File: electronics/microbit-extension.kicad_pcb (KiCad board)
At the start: 2 copper layers, 55.9 x 63.5 mm, 29 parts, among them J1 microbit_edge_connector, SW1 SW_DIP_x01, SW2 SW_DIP_x01, SW3 SW_DIP_x01, SW4 SW_DIP_x01, U1 LD1117S33CTR

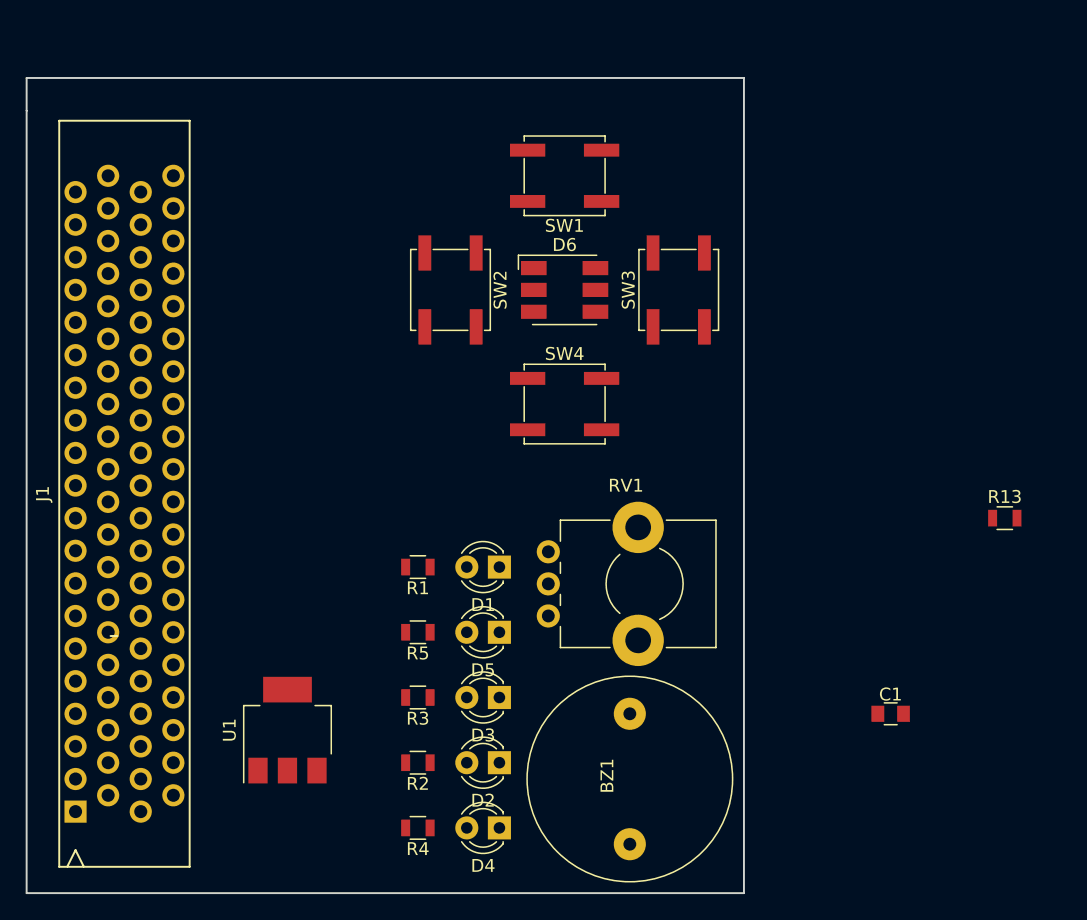
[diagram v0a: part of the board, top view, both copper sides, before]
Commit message: more layouting
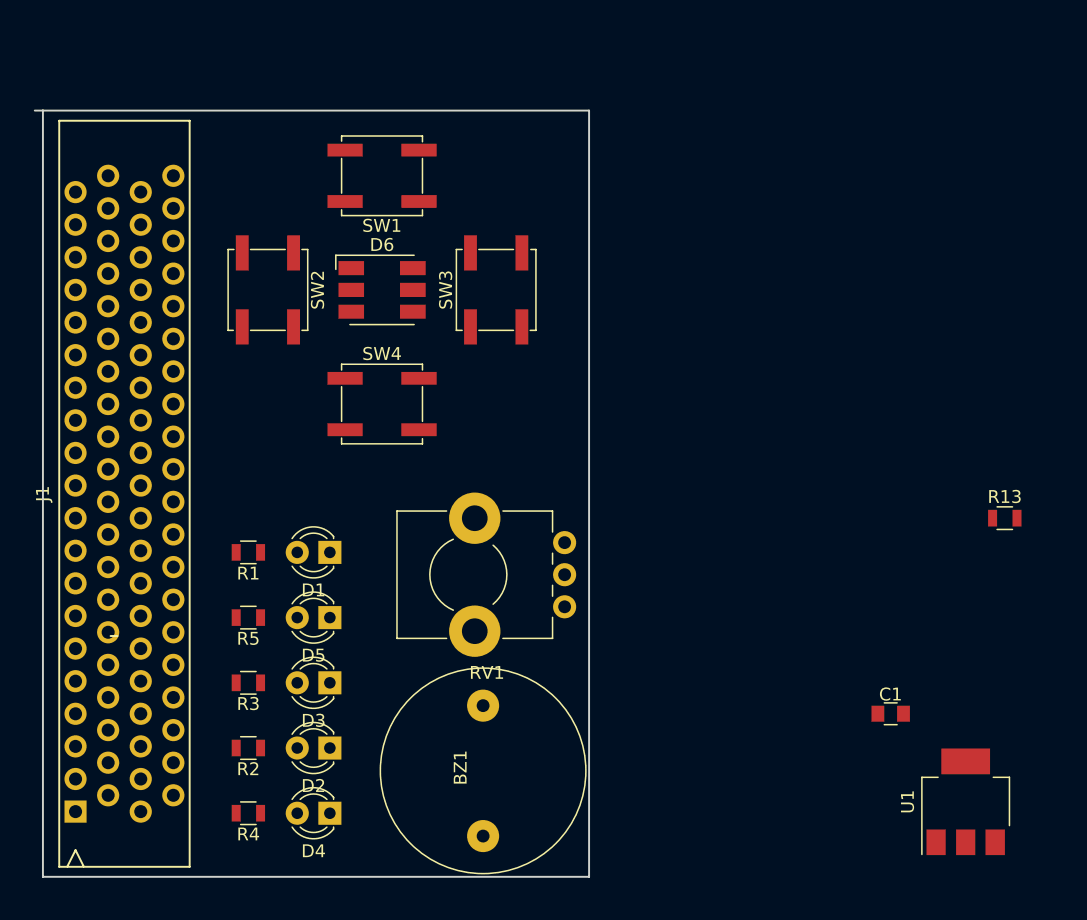
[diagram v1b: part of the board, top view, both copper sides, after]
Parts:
- moved U1 53.1 mm to (116.3, 122.4)
- moved D6 14.2 mm to (70.9, 82.5)
- moved SW1 14.2 mm to (70.9, 73.7)
- moved SW2 14.2 mm to (62.0, 82.5)
- moved SW3 14.2 mm to (79.8, 82.5)
- moved SW4 14.2 mm to (70.9, 91.4)
- moved D1 13.3 mm to (66.8, 103.0)
- moved D2 13.3 mm to (66.8, 118.2)
- moved D3 13.3 mm to (66.8, 113.2)
- moved D4 13.3 mm to (66.8, 123.3)
- moved D5 13.3 mm to (66.8, 108.1)
- moved R1 13.3 mm to (60.5, 103.0)
- moved R2 13.3 mm to (60.5, 118.2)
- moved R3 13.3 mm to (60.5, 113.2)
- moved R4 13.3 mm to (60.5, 123.3)
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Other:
- board size 55.9 x 63.5 mm -> 43.2 x 59.7 mm
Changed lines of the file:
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@@
     (links 78)
     (no_connects 78)
-    (area 43.104999 65.964999 99.135001 129.615001)
+    (area 43.739999 68.504999 87.070001 128.345001)
     (thickness 1.6)
     (drawings 5)
@@
   )
   (module Buzzers_Beepers:BUZZER (layer F.Cu)
-    (at 90.17 120.65 90)
+    (at 78.74 120.015 90)
     (fp_text reference BZ1 (at 0.24892 -1.75006 90) (layer F.SilkS)
       (effects (font (size 1 1) (thickness 0.15)))
@@
   )
   (module LEDs:LED_D3.0mm (layer F.Cu)
-    (at 80.01 104.14 180)
+    (at 66.802 102.997 180)
     (descr "LED, diameter 3.0mm, 2 pins")
     (tags "LED diameter 3.0mm 2 pins")
@@
   )
   (module LEDs:LED_D3.0mm (layer F.Cu)
-    (at 80.01 119.38 180)
+    (at 66.802 118.237 180)
     (descr "LED, diameter 3.0mm, 2 pins")
     (tags "LED diameter 3.0mm 2 pins")
@@
   )
   (module LEDs:LED_D3.0mm (layer F.Cu)
-    (at 80.01 114.3 180)
+    (at 66.802 113.157 180)
     (descr "LED, diameter 3.0mm, 2 pins")
     (tags "LED diameter 3.0mm 2 pins")
@@
   )
   (module LEDs:LED_D3.0mm (layer F.Cu)
-    (at 80.01 124.46 180)
+    (at 66.802 123.317 180)
     (descr "LED, diameter 3.0mm, 2 pins")
     (tags "LED diameter 3.0mm 2 pins")
@@
   )
   (module LEDs:LED_D3.0mm (layer F.Cu)
-    (at 80.01 109.22 180)
+    (at 66.802 108.077 180)
     (descr "LED, diameter 3.0mm, 2 pins")
     (tags "LED diameter 3.0mm 2 pins")
@@
   )
   (module LEDs:LED_RGB_5050-6 (layer F.Cu)
-    (at 85.09 82.55)
+    (at 70.866 82.55)
     (descr http://cdn.sparkfun.com/datasheets/Components/LED/5060BRG4.pdf)
     (tags "RGB LED 5050-6")
@@
   )
   (module Potentiometers:Potentiometer_Alps_RK09K_Horizontal (layer F.Cu)
-    (at 83.82 107.95)
+    (at 85.09 102.235 180)
     (descr "Potentiometer, horizontally mounted, Omeg PC16PU, Omeg PC16PU, Omeg PC16PU, Vishay/Spectrol 248GJ/249GJ Single, Vishay/Spectrol 248GJ/249GJ Single, Vishay/Spectrol 248GJ/249GJ Single, Vishay/Spectrol 248GH/249GH Single, Vishay/Spectrol 148/149 Single, Vishay/Spectrol 148/149 Single, Vishay/Spectrol 148/149 Single, Vishay/Spectrol 148A/149A Single with mounting plates, Vishay/Spectrol 148/149 Double, Vishay/Spectrol 148A/149A Double with mounting plates, Piher PC-16 Single, Piher PC-16 Single, Piher PC-16 Single, Piher PC-16SV Single, Piher PC-16 Double, Piher PC-16 Triple, Piher T16H Single, Piher T16L Single, Piher T16H Double, Alps RK163 Single, Alps RK163 Double, Alps RK097 Single, Alps RK097 Double, Bourns PTV09A-2 Single with mounting sleve Single, Bourns PTV09A-1 with mounting sleve Single, Bourns PRS11S Single, Alps RK09K Single with mounting sleve Single, Alps RK09K with mounting sleve Single, http://www.alps.com/prod/info/E/HTML/Potentiometer/RotaryPotentiometers/RK09K/RK09D1130C1B.html")
     (tags "Potentiometer horizontal  Omeg PC16PU  Omeg PC16PU  Omeg PC16PU  Vishay/Spectrol 248GJ/249GJ Single  Vishay/Spectrol 248GJ/249GJ Single  Vishay/Spectrol 248GJ/249GJ Single  Vishay/Spectrol 248GH/249GH Single  Vishay/Spectrol 148/149 Single  Vishay/Spectrol 148/149 Single  Vishay/Spectrol 148/149 Single  Vishay/Spectrol 148A/149A Single with mounting plates  Vishay/Spectrol 148/149 Double  Vishay/Spectrol 148A/149A Double with mounting plates  Piher PC-16 Single  Piher PC-16 Single  Piher PC-16 Single  Piher PC-16SV Single  Piher PC-16 Double  Piher PC-16 Triple  Piher T16H Single  Piher T16L Single  Piher T16H Double  Alps RK163 Single  Alps RK163 Double  Alps RK097 Single  Alps RK097 Double  Bourns PTV09A-2 Single with mounting sleve Single  Bourns PTV09A-1 with mounting sleve Single  Bourns PRS11S Single  Alps RK09K Single with mounting sleve Single  Alps RK09K with mounting sleve Single")
-    (fp_text reference RV1 (at 6.05 -10.15) (layer F.SilkS)
-      (effects (font (size 1 1) (thickness 0.15)))
-    )
-    (fp_text value POT (at 6.05 5.15) (layer F.Fab)
+    (fp_text reference RV1 (at 6.05 -10.15 180) (layer F.SilkS)
+      (effects (font (size 1 1) (thickness 0.15)))
+    )
+    (fp_text value POT (at 6.05 5.15 180) (layer F.Fab)
       (effects (font (size 1 1) (thickness 0.15)))
     )
@@
     (fp_line (start 13.25 4.15) (end 13.25 -9.15) (layer F.CrtYd) (width 0.05))
     (fp_line (start 13.25 -9.15) (end -1.15 -9.15) (layer F.CrtYd) (width 0.05))
-    (pad 3 thru_hole circle (at 0 -5) (size 1.8 1.8) (drill 1) (layers *.Cu *.Mask)
+    (pad 3 thru_hole circle (at 0 -5 180) (size 1.8 1.8) (drill 1) (layers *.Cu *.Mask)
       (net 2 +3V3))
-    (pad 2 thru_hole circle (at 0 -2.5) (size 1.8 1.8) (drill 1) (layers *.Cu *.Mask)
+    (pad 2 thru_hole circle (at 0 -2.5 180) (size 1.8 1.8) (drill 1) (layers *.Cu *.Mask)
       (net 37 /AI0))
-    (pad 1 thru_hole circle (at 0 0) (size 1.8 1.8) (drill 1) (layers *.Cu *.Mask)
-      (net 4 GND))
-    (pad 0 np_thru_hole circle (at 7 -6.9) (size 4 4) (drill 2) (layers *.Cu *.Mask))
-    (pad 0 np_thru_hole circle (at 7 1.9) (size 4 4) (drill 2) (layers *.Cu *.Mask))
+    (pad 1 thru_hole circle (at 0 0 180) (size 1.8 1.8) (drill 1) (layers *.Cu *.Mask)
+      (net 4 GND))
+    (pad 0 np_thru_hole circle (at 7 -6.9 180) (size 4 4) (drill 2) (layers *.Cu *.Mask))
+    (pad 0 np_thru_hole circle (at 7 1.9 180) (size 4 4) (drill 2) (layers *.Cu *.Mask))
     (model Potentiometers.3dshapes/Potentiometer_Alps_RK09K_Horizontal.wrl
       (at (xyz 0 0 0))
@@
   )
   (module TO_SOT_Packages_SMD:SOT-223 (layer F.Cu)
-    (at 63.5 116.84 90)
+    (at 116.332 122.428 90)
     (descr "module CMS SOT223 4 pins")
     (tags "CMS SOT")
@@
   )
   (module Resistors_SMD:R_0805 (layer F.Cu)
-    (at 73.66 104.14 180)
+    (at 60.452 102.997 180)
     (descr "Resistor SMD 0805, reflow soldering, Vishay (see dcrcw.pdf)")
     (tags "resistor 0805")
@@
   )
   (module Resistors_SMD:R_0805 (layer F.Cu)
-    (at 73.66 119.38 180)
+    (at 60.452 118.237 180)
     (descr "Resistor SMD 0805, reflow soldering, Vishay (see dcrcw.pdf)")
     (tags "resistor 0805")
@@
   )
   (module Resistors_SMD:R_0805 (layer F.Cu)
-    (at 73.66 114.3 180)
+    (at 60.452 113.157 180)
     (descr "Resistor SMD 0805, reflow soldering, Vishay (see dcrcw.pdf)")
     (tags "resistor 0805")
@@
   )
   (module Resistors_SMD:R_0805 (layer F.Cu)
-    (at 73.66 124.46 180)
+    (at 60.452 123.317 180)
     (descr "Resistor SMD 0805, reflow soldering, Vishay (see dcrcw.pdf)")
     (tags "resistor 0805")
@@
   )
   (module Resistors_SMD:R_0805 (layer F.Cu)
-    (at 73.66 109.22 180)
+    (at 60.452 108.077 180)
     (descr "Resistor SMD 0805, reflow soldering, Vishay (see dcrcw.pdf)")
     (tags "resistor 0805")
@@
   )
   (module Buttons_Switches_SMD:SW_SPST_EVPBF (layer F.Cu)
-    (at 85.09 73.66 180)
+    (at 70.866 73.66 180)
     (descr "Light Touch Switch")
     (attr smd)
@@
   )
   (module Buttons_Switches_SMD:SW_SPST_EVPBF (layer F.Cu)
-    (at 76.2 82.55 270)
+    (at 61.976 82.55 270)
     (descr "Light Touch Switch")
     (attr smd)
@@
   )
   (module Buttons_Switches_SMD:SW_SPST_EVPBF (layer F.Cu)
-    (at 93.98 82.55 90)
+    (at 79.756 82.55 90)
     (descr "Light Touch Switch")
     (attr smd)
@@
   )
   (module Buttons_Switches_SMD:SW_SPST_EVPBF (layer F.Cu)
-    (at 85.09 91.44)
+    (at 70.866 91.44)
     (descr "Light Touch Switch")
     (attr smd)
@@
     )
   )
-  (gr_line (start 43.18 66.04) (end 43.18 68.58) (angle 90) (layer Edge.Cuts) (width 0.15))
-  (gr_line (start 99.06 66.04) (end 43.18 66.04) (angle 90) (layer Edge.Cuts) (width 0.15))
-  (gr_line (start 99.06 129.54) (end 99.06 66.04) (angle 90) (layer Edge.Cuts) (width 0.15))
-  (gr_line (start 43.18 129.54) (end 99.06 129.54) (angle 90) (layer Edge.Cuts) (width 0.15))
-  (gr_line (start 43.18 68.58) (end 43.18 129.54) (angle 90) (layer Edge.Cuts) (width 0.15))
+  (gr_line (start 44.45 68.58) (end 43.815 68.58) (angle 90) (layer Edge.Cuts) (width 0.15))
+  (gr_line (start 44.45 128.27) (end 44.45 68.58) (angle 90) (layer Edge.Cuts) (width 0.15))
+  (gr_line (start 86.995 128.27) (end 44.45 128.27) (angle 90) (layer Edge.Cuts) (width 0.15))
+  (gr_line (start 86.995 68.58) (end 86.995 128.27) (angle 90) (layer Edge.Cuts) (width 0.15))
+  (gr_line (start 44.45 68.58) (end 86.995 68.58) (angle 90) (layer Edge.Cuts) (width 0.15))
 )
